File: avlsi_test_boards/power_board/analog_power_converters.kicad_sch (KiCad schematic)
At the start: 15 parts, among them U5 TLV1117LV18DCYR, U6 TLV75709PDBV, U7 TLV1117LV25DCYR, U8 TLV1117LV33DCYR

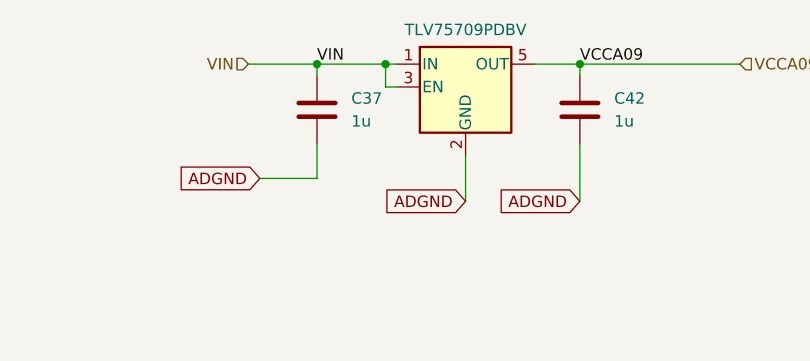
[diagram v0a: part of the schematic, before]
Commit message: more changes
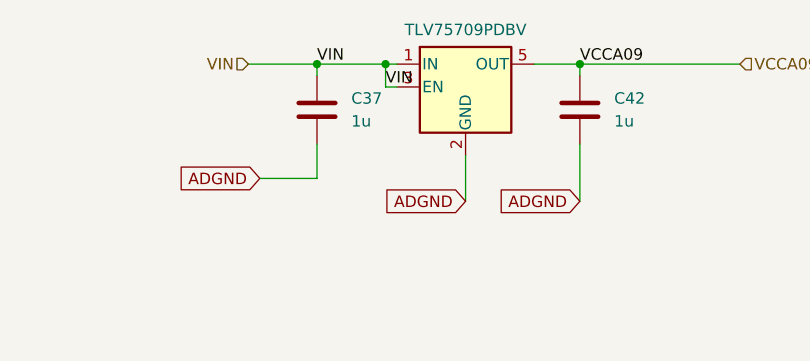
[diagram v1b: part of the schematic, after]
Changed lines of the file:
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@@
+	)
+	(label "VIN"
+		(at 107.95 31.75 0)
+		(fields_autoplaced yes)
+		(effects
+			(font
+				(size 1.27 1.27)
+			)
+			(justify left bottom)
+		)
 	)
 	(label "VIN"

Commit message: Add partial changes
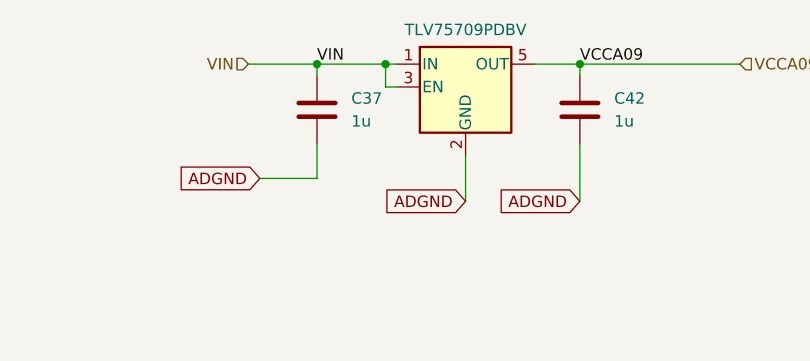
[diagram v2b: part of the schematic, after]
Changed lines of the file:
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@@
 	(label "VIN"
 		(at 100.33 29.21 0)
-		(fields_autoplaced yes)
-		(effects
-			(font
-				(size 1.27 1.27)
-			)
-			(justify left bottom)
-		)
-	)
-	(label "VIN"
-		(at 107.95 31.75 0)
-		(fields_autoplaced yes)
 		(effects
 			(font
@@
 	(label "VIN"
 		(at 157.48 78.74 0)
-		(fields_autoplaced yes)
 		(effects
 			(font
@@
 	(label "VCCA25"
 		(at 205.74 78.74 0)
-		(fields_autoplaced yes)
 		(effects
 			(font
@@
 	(label "VCCA12"
 		(at 73.66 78.74 0)
-		(fields_autoplaced yes)
 		(effects
 			(font
@@
 	(label "VIN"
 		(at 25.4 78.74 0)
-		(fields_autoplaced yes)
 		(effects
 			(font
@@
 	(label "VCCA18"
 		(at 72.39 115.57 0)
-		(fields_autoplaced yes)
 		(effects
 			(font
@@
 	(label "VIN"
 		(at 157.48 115.57 0)
-		(fields_autoplaced yes)
 		(effects
 			(font
@@
 	(label "VCCA33"
 		(at 205.74 115.57 0)
-		(fields_autoplaced yes)
 		(effects
 			(font
@@
 	(label "VIN"
 		(at 24.13 115.57 0)
-		(fields_autoplaced yes)
 		(effects
 			(font
@@
 	(label "VCCA09"
 		(at 129.54 29.21 0)
-		(fields_autoplaced yes)
 		(effects
 			(font
@@
 		(shape input)
 		(at 99.06 115.57 0)
-		(fields_autoplaced yes)
 		(effects
 			(font
@@
 		(shape input)
 		(at 231.14 115.57 0)
-		(fields_autoplaced yes)
 		(effects
 			(font
@@
 		(shape input)
 		(at 100.33 78.74 0)
-		(fields_autoplaced yes)
 		(effects
 			(font
@@
 		(shape input)
 		(at 147.32 29.21 0)
-		(fields_autoplaced yes)
 		(effects
 			(font
@@
 		(shape input)
 		(at 231.14 78.74 0)
-		(fields_autoplaced yes)
 		(effects
 			(font
@@
 		(shape input)
 		(at 92.71 29.21 180)
-		(fields_autoplaced yes)
-		(effects
-			(font
+		(effects
+			(font
